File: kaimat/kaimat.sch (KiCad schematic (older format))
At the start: 13 parts

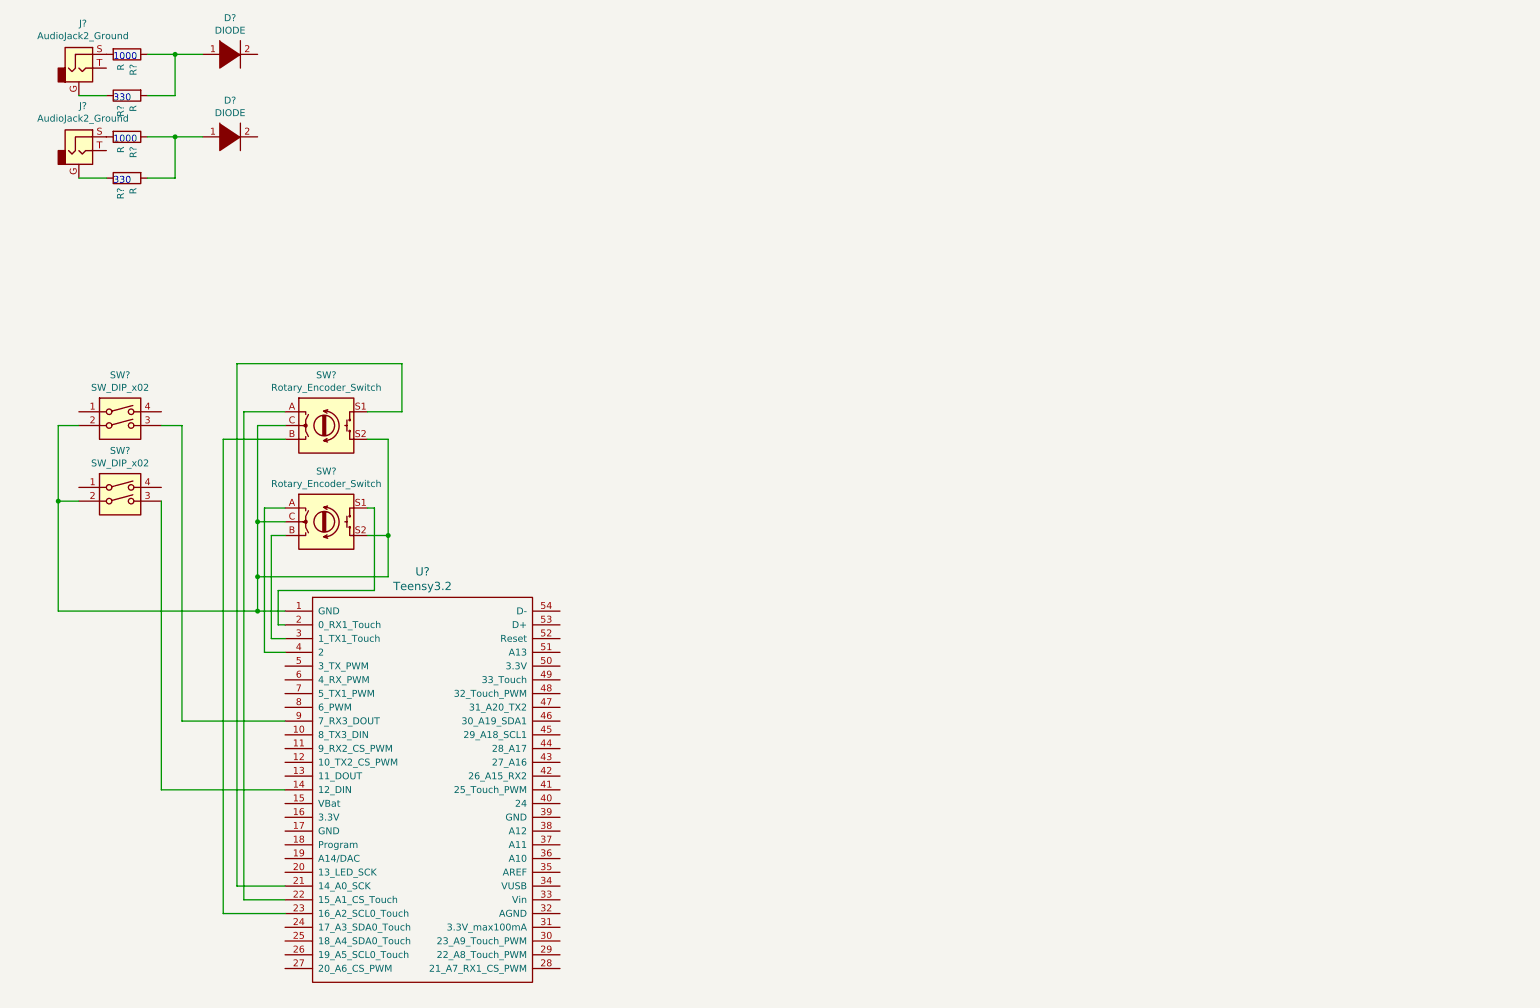
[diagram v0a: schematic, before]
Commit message: schematic finished
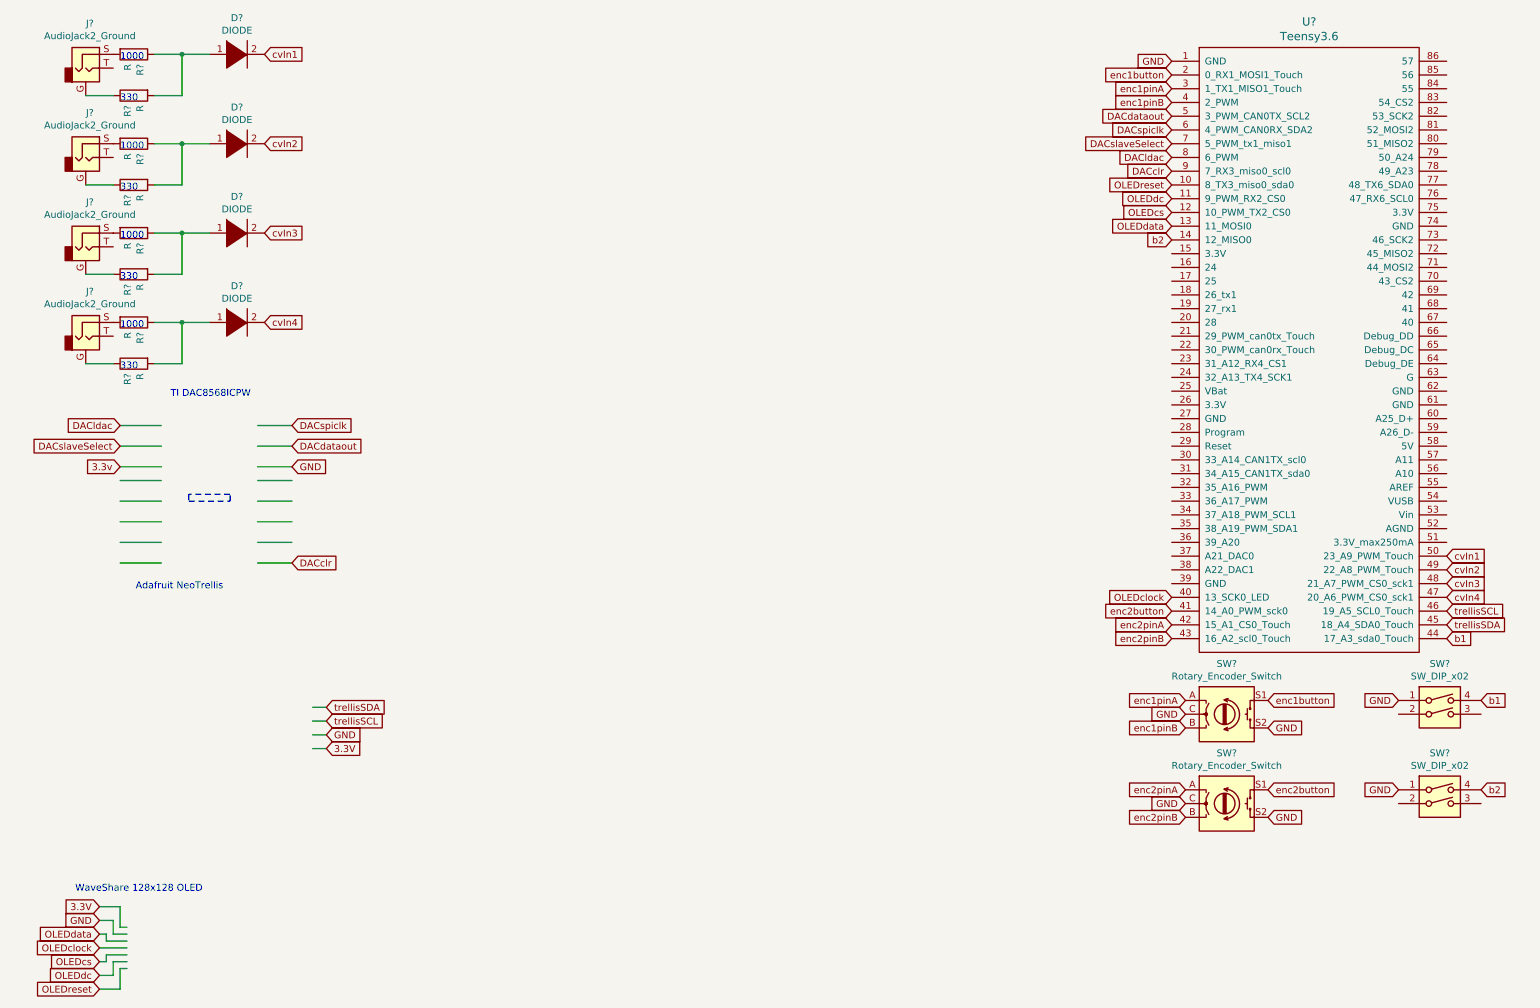
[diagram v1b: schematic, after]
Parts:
- removed U?: Teensy3.2, symbol teensy:Teensy3.2
- added D? (x2): DIODE, symbol pspice:DIODE
- added J? (x2): AudioJack2_Ground, symbol Connector:AudioJack2_Ground
- added R? (x4): R, symbol Device:R
- added U?: Teensy3.6, symbol teensy:Teensy3.6
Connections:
- net labels added: 3.3V, 3.3v, DACclr, DACdataout, DACldac, DACslaveSelect, DACspiclk, GND, OLEDclock, OLEDcs, OLEDdata, OLEDdc, OLEDreset, b1, b2, cvIn1, cvIn2, cvIn3, cvIn4, enc1button, enc1pinA, enc1pinB, enc2button, enc2pinA, enc2pinB, trellisSCL, trellisSDA
- wire segments 53 -> 59
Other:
- note added: "Adafruit NeoTrellis"
- note added: "TI DAC8568ICPW"
- note added: "WaveShare 128x128 OLED"
- moved on the sheet: D?, J?, R?, SW?
